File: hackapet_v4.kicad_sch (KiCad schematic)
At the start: 45 parts, among them J1 Conn_01x02_Socket, J4 USB_C_Receptacle_USB2.0_16P, J7 lipo, Q2 2N7002, SW1 SW_Push, SW2 SW_Push, SW3 SW_Push, SW4 SW_SPDT, U1 XC6206PxxxMR, U11 SRV05-4, U2 ESP-PSRAM32, U3 ESP32-S2-MINI-2, U4 BQ24075RGT

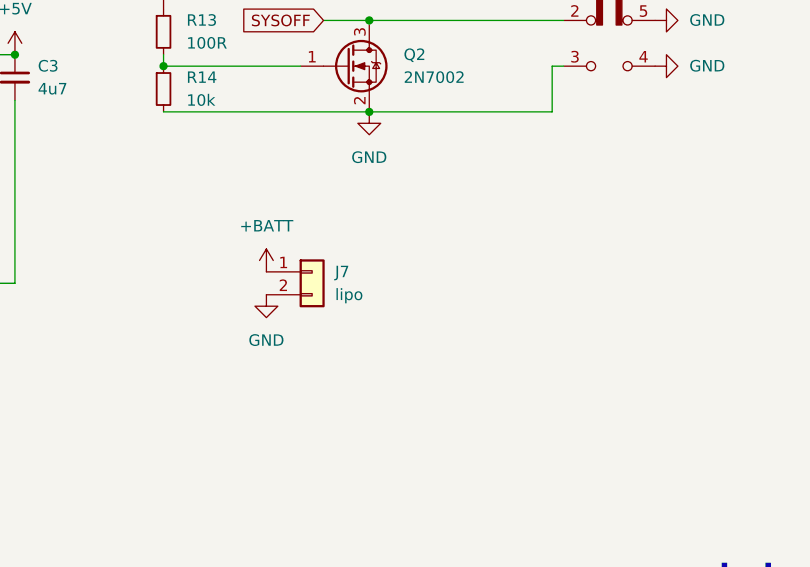
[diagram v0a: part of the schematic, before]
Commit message: final updates!
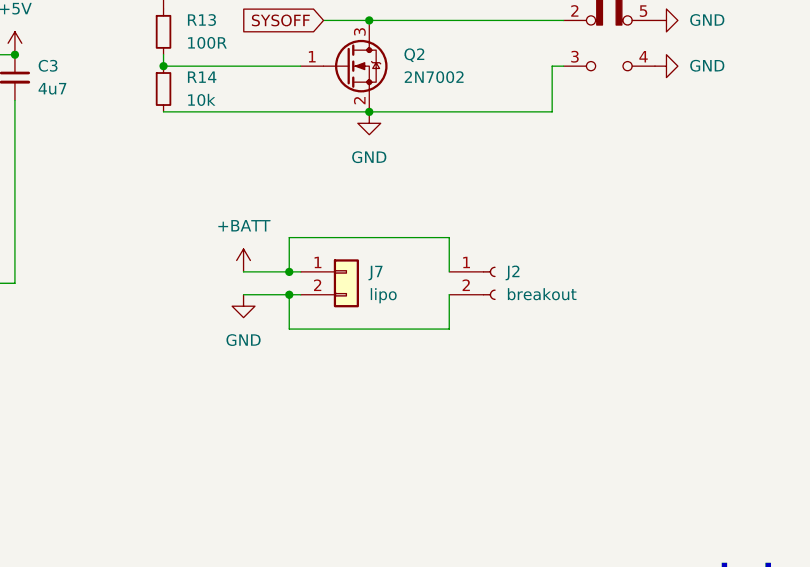
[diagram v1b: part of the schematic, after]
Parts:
- added J2: breakout, Connector_PinHeader_2.54mm:PinHeader_1x02_P2.54mm_Vertical_SMD_Pin1Left, symbol Connector:Conn_01x02_Socket
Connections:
- net +BATT: now also J2.1 (Pin_1)
- net GND: now also J2.2 (Pin_2)
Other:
- moved on the sheet: J7
